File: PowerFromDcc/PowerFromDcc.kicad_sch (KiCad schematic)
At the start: 15 parts, among them IC1 AP64060QWU-7, J1 DCC/J, J2 DCC/K, J3 5V, J4 Gnd, J5 DCC

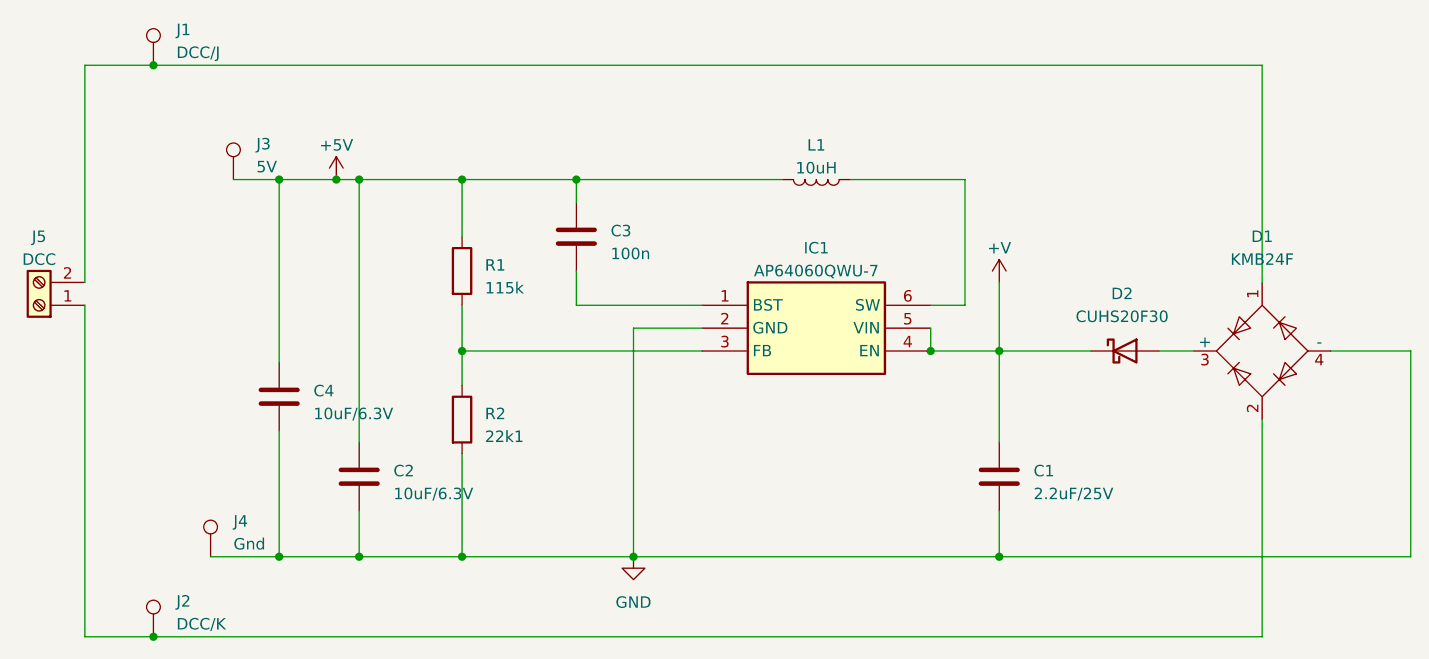
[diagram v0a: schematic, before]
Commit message: 04/12/24 20:52 Arrakis.local
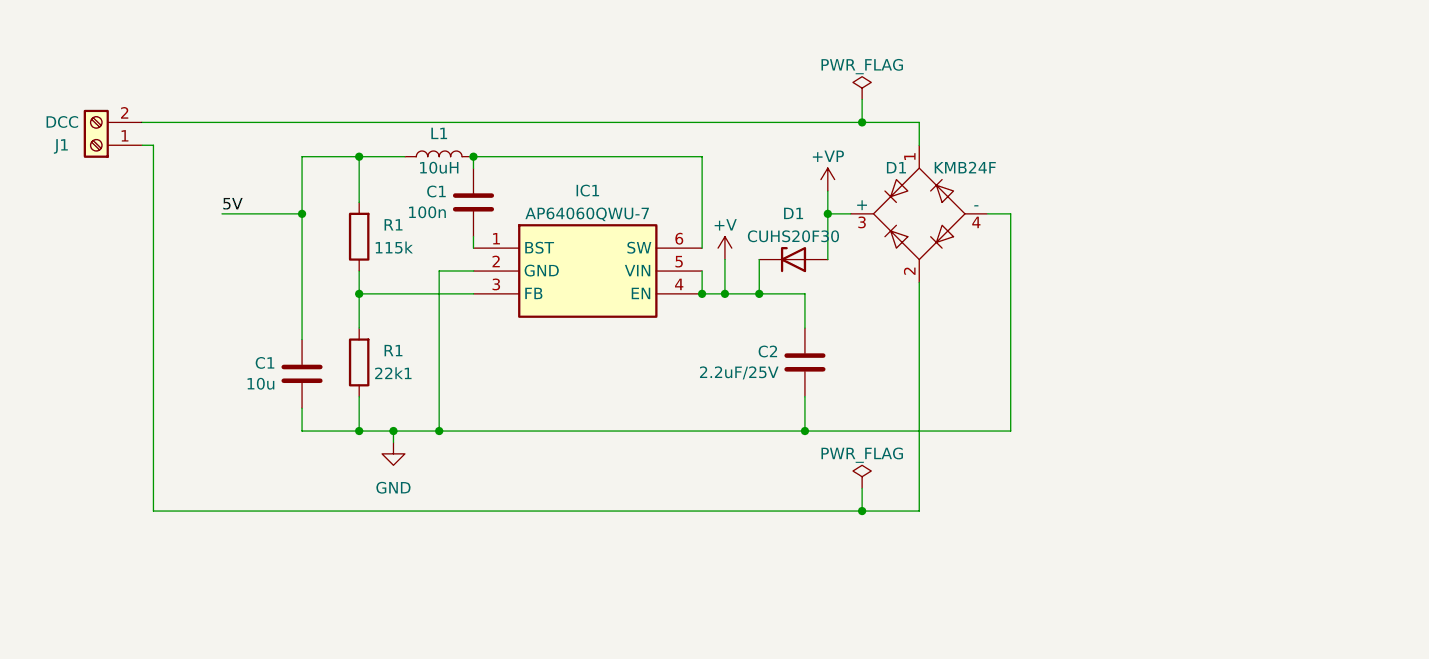
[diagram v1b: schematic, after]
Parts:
- removed C1: 2.2uF/25V, Capacitor_SMD:C_1206_3216Metric, symbol Device:C
- removed C3: 100n, Capacitor_SMD:C_1206_3216Metric, symbol Device:C
- removed C4: 10uF/6.3V, Capacitor_SMD:C_1206_3216Metric, symbol Device:C
- removed D1: KMB24F, Package_TO_SOT_SMD:TO-269AA, symbol Additional:KMB24F
- removed D2: CUHS20F30, Diode_SMD:D_1206_3216Metric, symbol Device:D_Schottky
- removed J1: DCC/J, TestPoint:TestPoint_Pad_D2.0mm, symbol Connector:TestPoint
- removed J2: DCC/K, TestPoint:TestPoint_Pad_D2.0mm, symbol Connector:TestPoint
- removed J3: 5V, TestPoint:TestPoint_Pad_D2.0mm, symbol Connector:TestPoint
- removed J4: Gnd, TestPoint:TestPoint_Pad_D2.0mm, symbol Connector:TestPoint
- removed J5: DCC, TerminalBlock_Phoenix:TerminalBlock_Phoenix_PT-1,5-2-3.5-H_1x02_P3.50mm_Horizontal, symbol Connector:Screw_Terminal_01x02
- removed R1: 115k, Resistor_SMD:R_1206_3216Metric, symbol Device:R
- removed R2: 22k1, Resistor_SMD:R_1206_3216Metric, symbol Device:R
- added C1: 10u, Capacitor_SMD:C_1206_3216Metric_Pad1.33x1.80mm_HandSolder, symbol Device:C
- added C1: 100n, Capacitor_SMD:C_1206_3216Metric_Pad1.33x1.80mm_HandSolder, symbol Device:C
- added D1: KMB24F, Package_TO_SOT_SMD:TO-269AA, symbol RP2040-Decoder_Additional_Symbols:KMB24F
- added D1: CUHS20F30, CUHS20F30:CUHS20F30H3F, symbol Device:D_Zener
- added J1: DCC, TerminalBlock_Phoenix:TerminalBlock_Phoenix_PT-1,5-2-3.5-H_1x02_P3.50mm_Horizontal, symbol Connector:Screw_Terminal_01x02
- added R1: 115k, Resistor_SMD:R_1206_3216Metric_Pad1.30x1.75mm_HandSolder, symbol Device:R
- added R1: 22k1, Resistor_SMD:R_1206_3216Metric_Pad1.30x1.75mm_HandSolder, symbol Device:R
- C2: value 10uF/6.3V -> 2.2uF/25V; footprint Capacitor_SMD:C_1206_3216Metric -> Capacitor_SMD:C_1206_3216Metric_Pad1.33x1.80mm_HandSolder
- IC1: footprint Package_TO_SOT_SMD:SOT-23-6 -> Package_TO_SOT_SMD:TSOT-23-6
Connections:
- net +V: now also C2.1, D1.1 (K), D1.2 (A), D1.3 (+)
- net GND: now also C1.2, D1.4 (-), R1.1
- net at IC1.1 (BST): now also C1.2
- net at IC1.3 (FB): now also R1.1, R1.2
- net at IC1.6 (SW): now also L1.2, C1.1; no longer L1.1
- removed net +5V: C2.1, L1.2
- new net: D1.1, J1.2 (Pin_2)
- new net: D1.2, J1.1 (Pin_1)
- new net 5V: C1.1, L1.1, R1.2
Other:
- title: DC powerfrom DCC -> (none)
